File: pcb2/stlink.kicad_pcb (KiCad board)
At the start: 4 copper layers, 44.5 x 33 mm, 37 parts, among them J1 USB_C_Receptacle_USB2.0-Conne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, J2 IDC 2x5, J3 Conn_01x05, Q1 S9013, U1 STM32F103CB, U3 AMS1117-3.3, Y1 8MHz

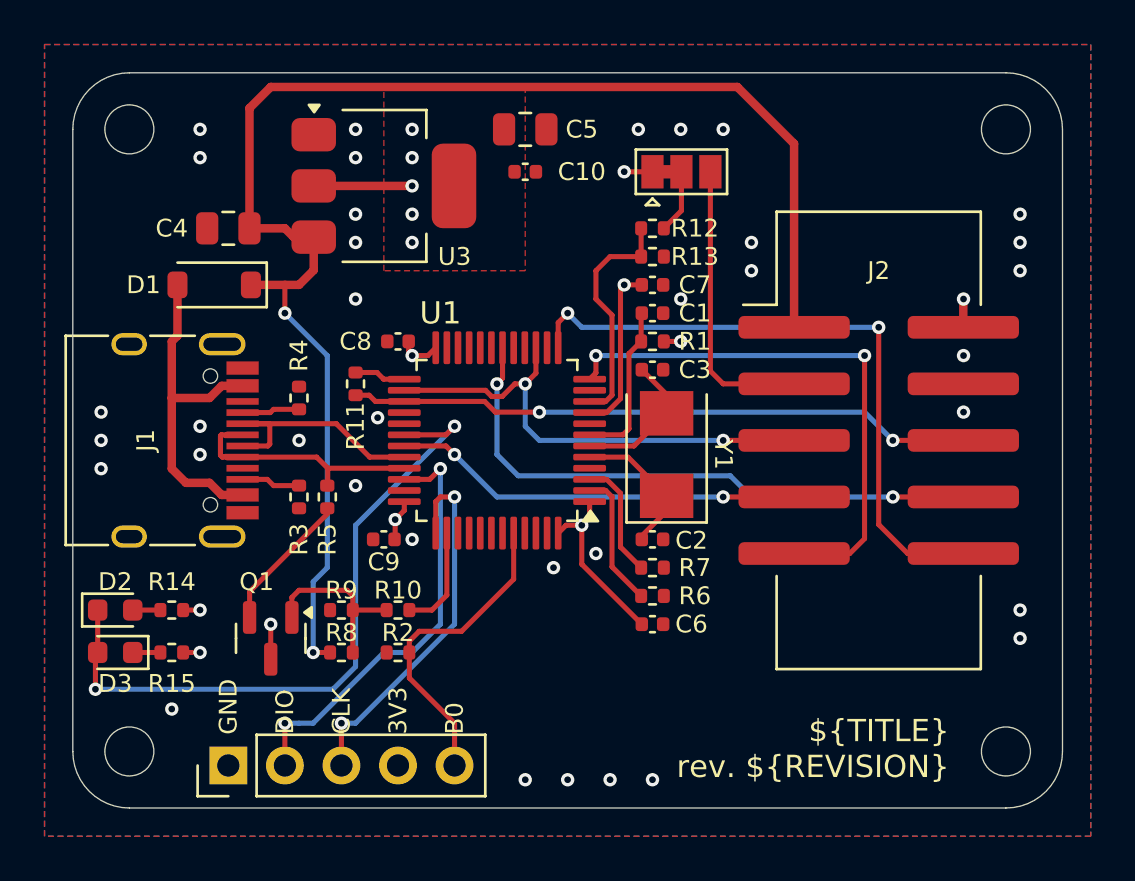
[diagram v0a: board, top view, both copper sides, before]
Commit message: Hmmmm
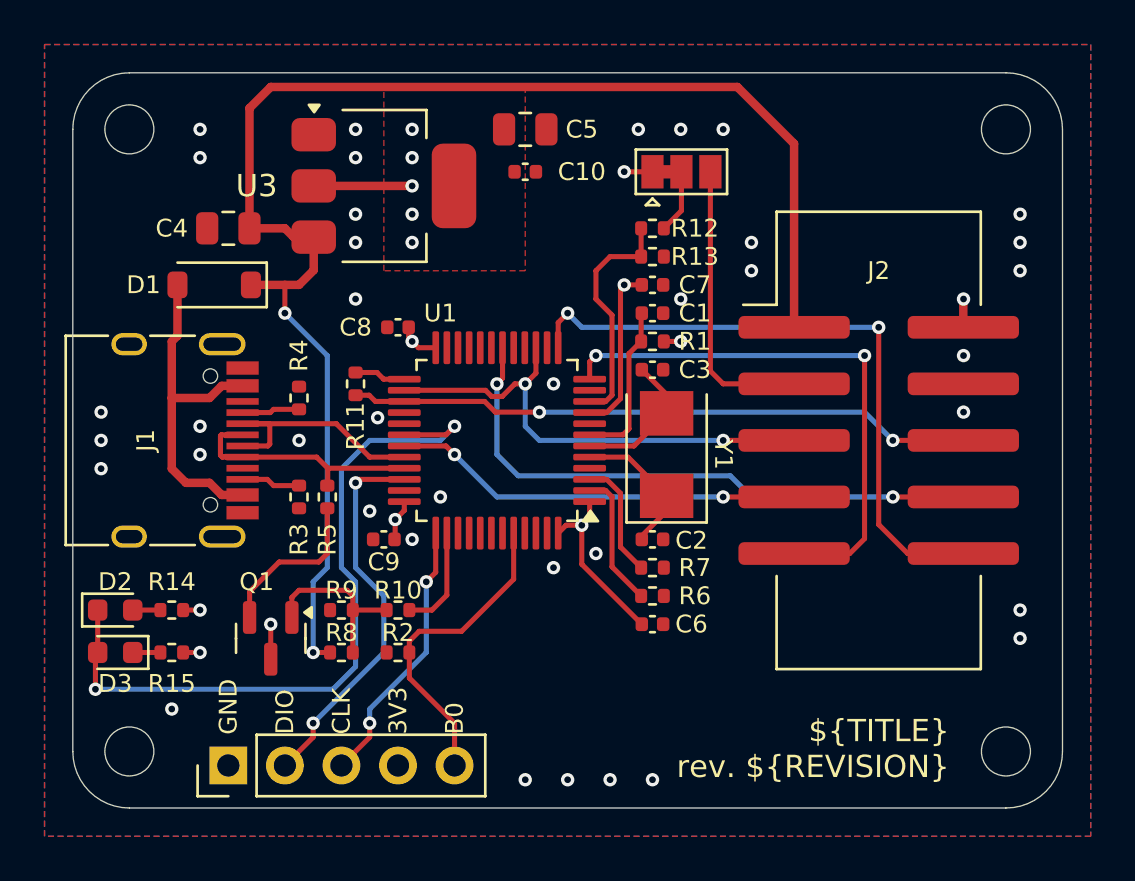
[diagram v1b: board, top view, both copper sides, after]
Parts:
- moved C8 0.64 mm to (116.2, 83.8)
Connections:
- R10 pad 2: Net-(Q1-B) -> Net-(Q1-PadB)
- R5 pad 2: Net-(Q1-E) -> Net-(Q1-PadE)
- R8 pad 1: Net-(Q1-B) -> Net-(Q1-PadB)
- R9 pad 2: Net-(Q1-B) -> Net-(Q1-PadB)
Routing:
- net Net-(Q1-PadB): track 0.00 -> 7.93 mm
- net Net-(Q1-B): track 7.93 -> 0.00 mm
- net Net-(Q1-PadE): track 0.00 -> 7.39 mm
- net Net-(Q1-E): track 6.35 -> 0.00 mm
- net CLK: track 16.9 -> 12.2 mm
- net LED: track 30.8 -> 33.1 mm
- net DIO: track 19.5 -> 17.3 mm
- net GND: vias 37 -> 39
